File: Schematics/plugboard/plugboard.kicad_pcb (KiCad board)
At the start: 2 copper layers, 35 parts, among them J1 Conn_01x01_Socket, J10 Conn_01x01_Socket, J11 Conn_01x01_Socket, J12 Conn_01x01_Socket, J13 Conn_01x01_Socket, J14 Conn_01x01_Socket, J15 Conn_01x01_Socket, J16 Conn_01x01_Socket, J17 Conn_01x01_Socket, J18 Conn_01x01_Socket, J19 Conn_01x01_Socket, J2 Conn_01x01_Socket, J20 Conn_01x01_Socket, J21 Conn_01x01_Socket, J22 Conn_01x01_Socket, J23 Conn_01x01_Socket, J24 Conn_01x01_Socket, J25 Conn_01x01_Socket, J26 Conn_01x01_Socket, J27 Conn_01x04, J3 Conn_01x01_Socket, J4 Conn_01x01_Socket, J5 Conn_01x01_Socket, J6 Conn_01x01_Socket, J7 Conn_01x01_Socket, J8 Conn_01x01_Socket, J9 Conn_01x01_Socket, U1 MCP23017_SP, U2 MCP23017_SP

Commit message: Plugboard PCB design done and send for manufacturing + a few edits
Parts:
- removed JP1, JP2, JP3, JP4, JP5, JP6: SolderJumper_3_Open, Jumper:SolderJumper-3_P1.3mm_Open_RoundedPad1.0x1.5mm_NumberLabels
- added J28: Conn_01x01_Socket, user_global_footprints:plugboard_test_socket, F.Cu at (37.7, 70.3)
- added J29: Conn_01x01_Socket, user_global_footprints:plugboard_test_socket, F.Cu at (255.3, 70.3)
- J1, J10, J11, J12, J13, J14, J15, J16, J17, J18, J19, J2, J20, J21, J22, J23, J24, J25, J26, J3, J4, J5, J6, J7, J8, J9: footprint Connector:Banana_Jack_1Pin -> user_global_footprints:plugboard_socket; moved to B.Cu
- J27: value Conn_01x04 -> Conn_01x04_Pin; footprint Connector_PinHeader_2.54mm:PinHeader_1x04_P2.54mm_Vertical -> user_global_footprints:PinHeader_1x04_P2.54mm_Vertical_SLIM
- U1, U2: value MCP23017_SP -> MCP23017_SO; footprint Package_DIP:DIP-28_W7.62mm -> user_global_footprints:SOIC-28W_7.5x17.9mm_P1.27mm_long_pads
- moved J1 224.3 mm to (250.5, 43.1), turned to 180 degrees
- moved J27 199.1 mm to (224.5, 65.2)
- moved J2 197.7 mm to (224.5, 43.1), turned to 180 degrees
- moved J18 185.0 mm to (250.5, 85.8), turned to 180 degrees
- moved J10 172.9 mm to (237.5, 63.8), turned to 180 degrees
- moved J3 171.7 mm to (198.5, 43.1), turned to 180 degrees
- moved U2 155.4 mm to (185.5, 97.9)
- moved J4 146.7 mm to (172.5, 43.1), turned to 180 degrees
- moved J11 145.0 mm to (211.5, 63.8), turned to 180 degrees
- moved J19 128.7 mm to (224.5, 85.8), turned to 180 degrees
- moved J5 123.4 mm to (146.5, 43.1), turned to 180 degrees
- moved J12 117.5 mm to (185.5, 63.8), turned to 180 degrees
- moved J6 102.7 mm to (120.5, 43.1), turned to 180 degrees
- moved J20 100.1 mm to (198.5, 85.8), turned to 180 degrees
- moved U1 90.8 mm to (107.6, 97.9)
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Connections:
- J27 pad 1: SCK -> VSS
- J27 pad 2: SDA -> VDD
- J27 pad 3: VDD -> SDA
- J27 pad 4: VSS -> SCK
- U1 pad 1: /O -> /I
- U1 pad 15: Net-(JP1-C) -> VSS
- U1 pad 16: Net-(JP2-C) -> VDD
- U1 pad 17: Net-(JP3-C) -> VSS
- U1 pad 2: /A -> /J
- U1 pad 21: /Q -> /A
- U1 pad 22: /W -> /B
- U1 pad 23: /E -> /C
- U1 pad 24: /R -> /D
- U1 pad 25: /T -> /E
- U1 pad 26: /Z -> /F
- U1 pad 27: /U -> /G
- U1 pad 28: /I -> /H
- U1 pad 3: /S -> /K
- U1 pad 4: /D -> /L
- U1 pad 5: /F -> /M
- U1 pad 6: /G -> /N
- U1 pad 7: /H -> /O
- U1 pad 8: /J -> /P
- U2 pad 1: /M -> /Y
- U2 pad 15: Net-(JP4-C) -> VDD
- U2 pad 16: Net-(JP5-C) -> VDD
- U2 pad 17: Net-(JP6-C) -> VSS
- U2 pad 2: /L -> /Z
- U2 pad 21: /K -> /Q
- U2 pad 22: /P -> /R
- U2 pad 23: /Y -> /S
- U2 pad 24: /X -> /T
- U2 pad 25: /C -> /U
- U2 pad 27: /B -> /W
- U2 pad 28: /N -> /X
- U2 pad 3: unconnected-(U2-GPB2-Pad3) -> /BT
- U2 pad 4: unconnected-(U2-GPB3-Pad4) -> /LT
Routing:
- net /BT: track 0.00 -> 197.6 mm, vias 0 -> 4
- net VDD: track 0.00 -> 176.0 mm, vias 0 -> 4
- net /A: track 0.00 -> 166.9 mm, vias 0 -> 1
- net /P: track 0.00 -> 166.6 mm, vias 0 -> 2
- net SDA: track 0.00 -> 154.7 mm, vias 0 -> 2
- net SCK: track 0.00 -> 150.9 mm, vias 0 -> 2
- net /U: track 0.00 -> 135.1 mm, vias 0 -> 2
- net /E: track 0.00 -> 119.0 mm, vias 0 -> 1
- net /O: track 0.00 -> 102.9 mm, vias 0 -> 1
- net /Z: track 0.00 -> 99.1 mm
- net /Q: track 0.00 -> 94.4 mm, vias 0 -> 1
- net /D: track 0.00 -> 89.2 mm, vias 0 -> 1
- net /LT: track 0.00 -> 89.1 mm, vias 0 -> 2
- net /M: track 0.00 -> 88.0 mm, vias 0 -> 1
- net /C: track 0.00 -> 73.9 mm, vias 0 -> 1
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- added copper zone on B.Cu, net VSS
- added copper zone on F.Cu, net VSS
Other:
- board outline added: 230 x 73 mm
- board text added: "CUED | lzb23 Enigma Plugboard v1.0 5/02/24"
- board text added: "SCL"
- board text added: "SDA"
- board text added: "THIS SIDE INTO MACHINE"
- board text added: "VDD"
- board text added: "VSS"
- board text added: "https://github.com/lbligh/enigma-iib-lzb23"

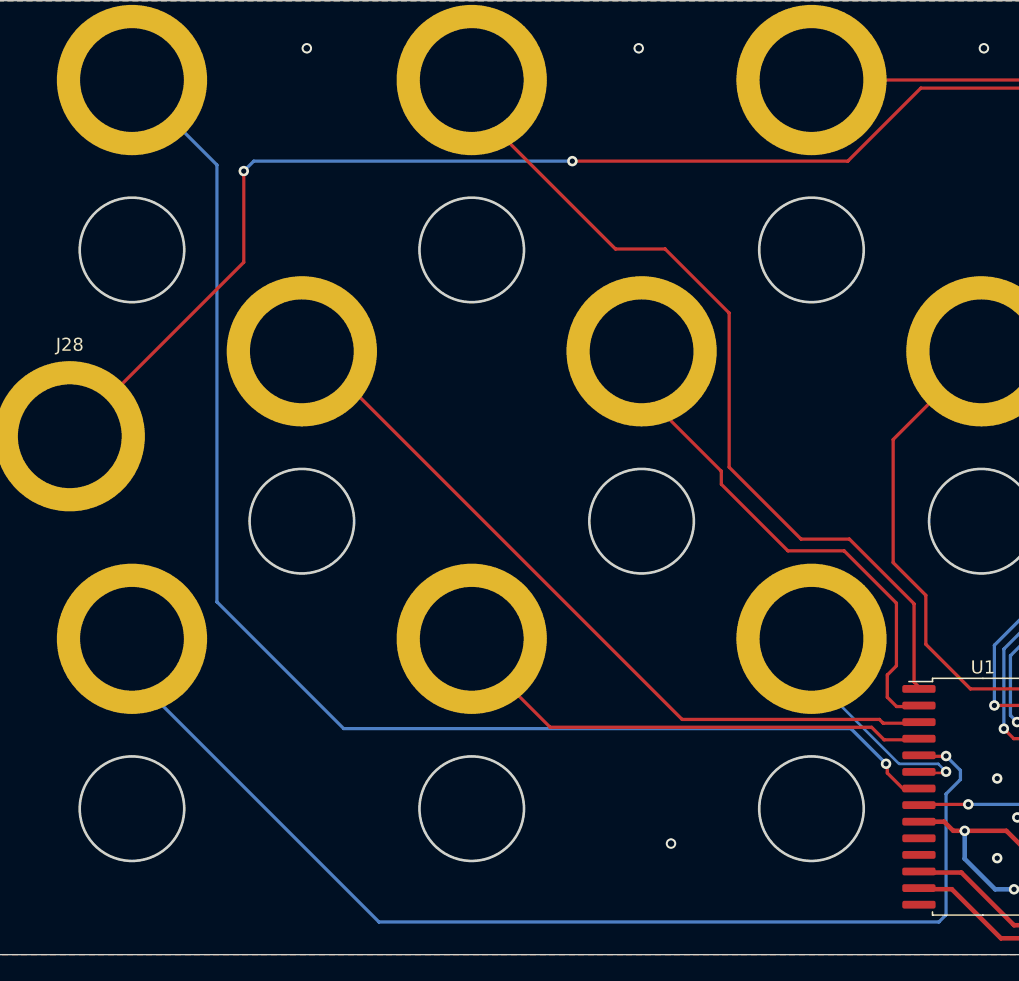
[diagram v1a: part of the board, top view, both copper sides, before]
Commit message: Final Commit
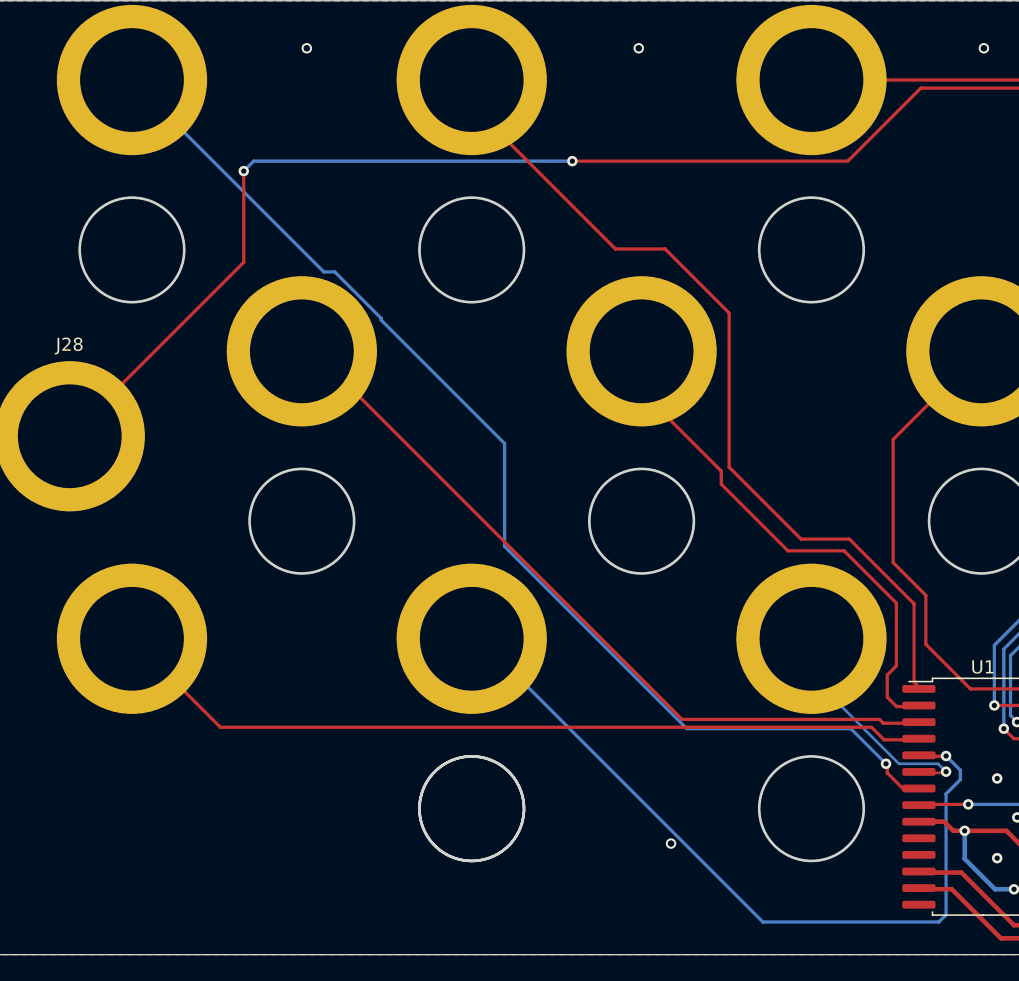
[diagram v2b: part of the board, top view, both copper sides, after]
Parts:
- moved J26 26.0 mm to (68.5, 85.8)
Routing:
- net /L: track 38.1 -> 66.4 mm
- net /M: track 88.0 -> 61.2 mm
- net /O: track 102.9 -> 88.0 mm
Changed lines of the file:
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@@
   )
   (footprint "user_global_footprints:plugboard_socket" (layer "B.Cu")
-    (at 42.5 85.83 180)
+    (at 68.5 85.83 180)
     (property "Letter" "Letter: L")
     (property "Sheetfile" "plugboard.kicad_sch")
@@
     (pad "" np_thru_hole circle (at 0 -13 180) (size 8 8) (drill 8) (layers "F&B.Cu" "*.Mask")
       (clearance 2))
-    (pad "1" thru_hole circle (at 0 0 180) (size 11.5 11.5) (drill 7.94) (layers "*.Cu" "*.Mask")
+    (pad "1" thru_hole circle (at 26 0 180) (size 11.5 11.5) (drill 7.94) (layers "*.Cu" "*.Mask")
       (net 25 "/L") (pinfunction "Pin_1") (pintype "passive") (clearance 0.2))
   )
@@
   (segment (start 100.205378 95.394622) (end 100.3 95.489244) (width 0.25) (layer "F.Cu") (net 9))
   (via (at 100.205378 95.394622) (size 0.8) (drill 0.4) (layers "F.Cu" "B.Cu") (net 9))
+  (segment (start 61.575 61.448) (end 61.575 61.313652) (width 0.25) (layer "B.Cu") (net 9))
+  (segment (start 84.958 92.705) (end 71.016348 78.763348) (width 0.25) (layer "B.Cu") (net 9))
+  (segment (start 57.185 57.755) (end 42.5 43.07) (width 0.25) (layer "B.Cu") (net 9))
   (segment (start 100.205378 95.394622) (end 97.515756 92.705) (width 0.25) (layer "B.Cu") (net 9))
-  (segment (start 49 49.57) (end 42.5 43.07) (width 0.25) (layer "B.Cu") (net 9))
-  (segment (start 49 83) (end 49 49.57) (width 0.25) (layer "B.Cu") (net 9))
-  (segment (start 58.705 92.705) (end 49 83) (width 0.25) (layer "B.Cu") (net 9))
-  (segment (start 97.515756 92.705) (end 58.705 92.705) (width 0.25) (layer "B.Cu") (net 9))
+  (segment (start 97.515756 92.705) (end 84.958 92.705) (width 0.25) (layer "B.Cu") (net 9))
+  (segment (start 71.016348 78.763348) (end 71.016348 70.889348) (width 0.25) (layer "B.Cu") (net 9))
+  (segment (start 58.016348 57.755) (end 57.185 57.755) (width 0.25) (layer "B.Cu") (net 9))
+  (segment (start 61.575 61.313652) (end 58.016348 57.755) (width 0.25) (layer "B.Cu") (net 9))
+  (segment (start 71.016348 70.889348) (end 61.575 61.448) (width 0.25) (layer "B.Cu") (net 9))
   (segment (start 112.5 98.635) (end 111.115 98.635) (width 0.25) (layer "F.Cu") (net 10))
   (segment (start 111.115 98.635) (end 110.25 99.5) (width 0.25) (layer "F.Cu") (net 10))
@@
   (segment (start 94.5 88.7) (end 94.5 85.83) (width 0.2) (layer "B.Cu") (net 24))
   (segment (start 101.2 95.4) (end 94.5 88.7) (width 0.2) (layer "B.Cu") (net 24))
-  (segment (start 99.1 92.6) (end 100.06 93.56) (width 0.25) (layer "F.Cu") (net 25))
-  (segment (start 74.5 92.6) (end 99.1 92.6) (width 0.25) (layer "F.Cu") (net 25))
-  (segment (start 68.5 86.6) (end 74.5 92.6) (width 0.25) (layer "F.Cu") (net 25))
-  (segment (start 68.5 85.83) (end 68.5 86.6) (width 0.25) (layer "F.Cu") (net 25))
-  (segment (start 100.06 93.56) (end 102.945 93.56) (width 0.25) (layer "F.Cu") (net 25))
+  (segment (start 49.27 92.6) (end 42.5 85.83) (width 0.25) (layer "F.Cu") (net 25))
+  (segment (start 100.06 93.56) (end 99.1 92.6) (width 0.25) (layer "F.Cu") (net 25))
+  (segment (start 99.1 92.6) (end 49.27 92.6) (width 0.25) (layer "F.Cu") (net 25))
+  (segment (start 102.945 93.56) (end 100.06 93.56) (width 0.25) (layer "F.Cu") (net 25))
+  (segment (start 42.5 88.6) (end 42.5 85.83) (width 0.25) (layer "B.Cu") (net 25))
   (segment (start 102.95 94.825) (end 104.775 94.825) (width 0.25) (layer "F.Cu") (net 26))
   (segment (start 104.775 94.825) (end 104.8 94.8) (width 0.25) (layer "F.Cu") (net 26))
+  (segment (start 68.5 85.83) (end 68.5 86.6) (width 0.25) (layer "F.Cu") (net 26))
   (via (at 104.8 94.8) (size 0.8) (drill 0.4) (layers "F.Cu" "B.Cu") (net 26))
+  (segment (start 104.8 97.7) (end 104.8 106.95) (width 0.25) (layer "B.Cu") (net 26))
+  (segment (start 69.105305 85.83) (end 68.5 85.83) (width 0.25) (layer "B.Cu") (net 26))
+  (segment (start 105.9 95.9) (end 105.9 96.6) (width 0.25) (layer "B.Cu") (net 26))
   (segment (start 105.9 96.6) (end 104.8 97.7) (width 0.25) (layer "B.Cu") (net 26))
-  (segment (start 104.8 97.7) (end 104.8 106.95) (width 0.25) (layer "B.Cu") (net 26))
-  (segment (start 105.9 95.9) (end 105.9 96.6) (width 0.25) (layer "B.Cu") (net 26))
-  (segment (start 104.25 107.5) (end 61.4 107.5) (width 0.25) (layer "B.Cu") (net 26))
   (segment (start 104.8 106.95) (end 104.25 107.5) (width 0.25) (layer "B.Cu") (net 26))
-  (segment (start 61.4 107.5) (end 42.5 88.6) (width 0.25) (layer "B.Cu") (net 26))
-  (segment (start 42.5 88.6) (end 42.5 85.83) (width 0.25) (layer "B.Cu") (net 26))
   (segment (start 104.8 94.8) (end 105.9 95.9) (width 0.25) (layer "B.Cu") (net 26))
+  (segment (start 104.25 107.5) (end 90.775305 107.5) (width 0.25) (layer "B.Cu") (net 26))
+  (segment (start 90.775305 107.5) (end 69.105305 85.83) (width 0.25) (layer "B.Cu") (net 26))
   (segment (start 176.024952 106.725048) (end 179.03 103.72) (width 0.35) (layer "F.Cu") (net 27))
   (segment (start 176.024952 106.774952) (end 176.024952 106.725048) (width 0.35) (layer "F.Cu") (net 27))
